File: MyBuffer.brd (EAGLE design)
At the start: 137.5 x 110 mm, 102 parts, among them Q1 BD140, Q2 BD139, Q3 BD140, Q4 BD139, Q5 BD139, Q6 BD139, T10 BD140, T11 BD139, T12 BD140, T13 BD139, T14 BD140, T17 BD139, T18 BD140, T9 BD139

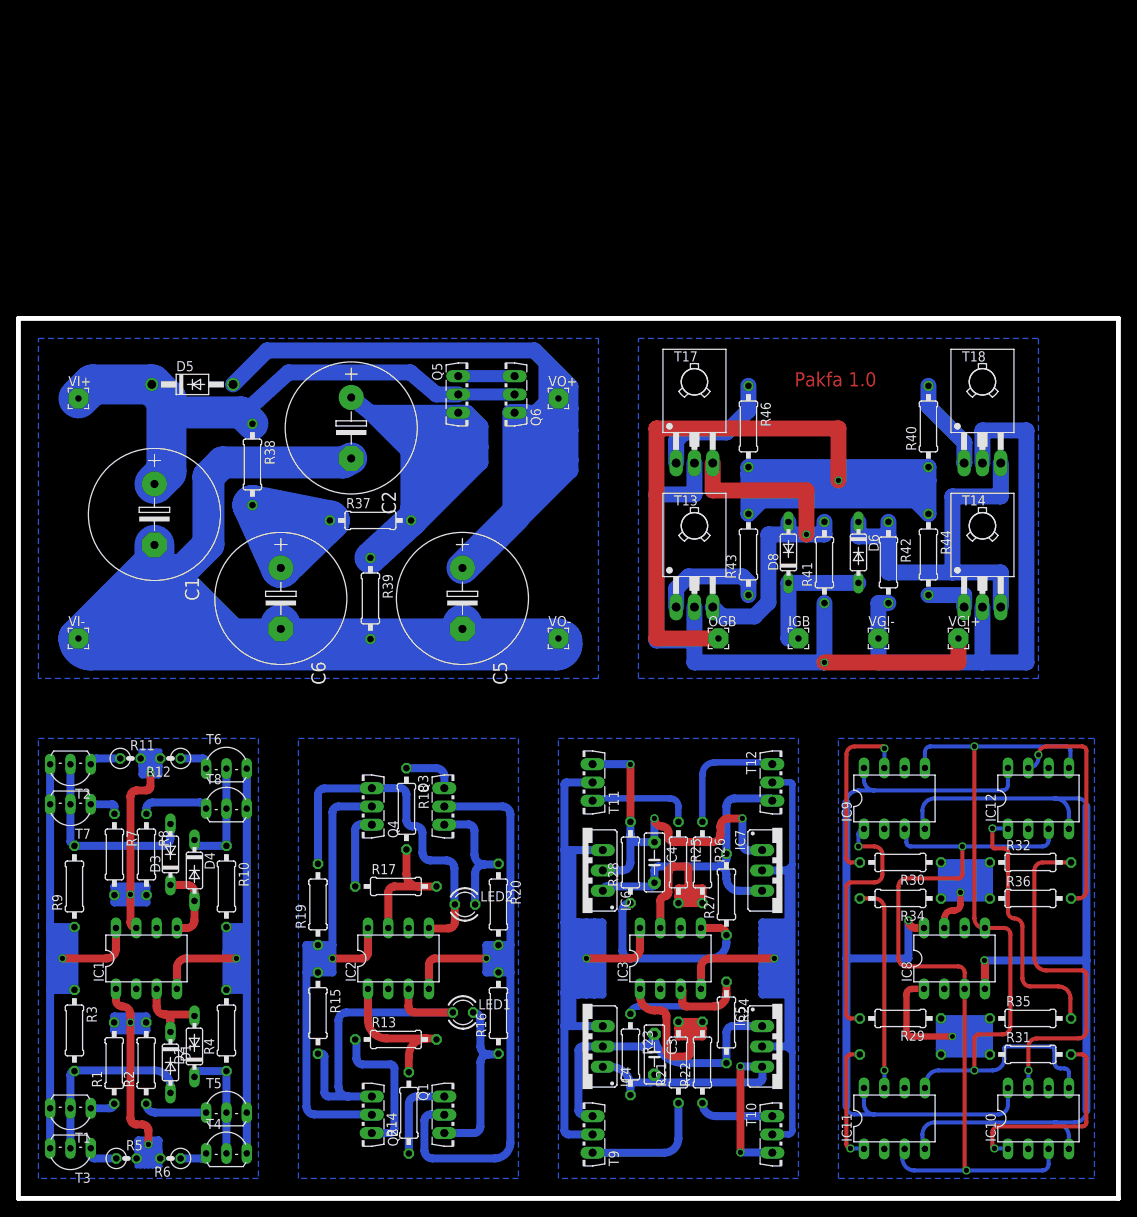
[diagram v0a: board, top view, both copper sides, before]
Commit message: Initial Commit
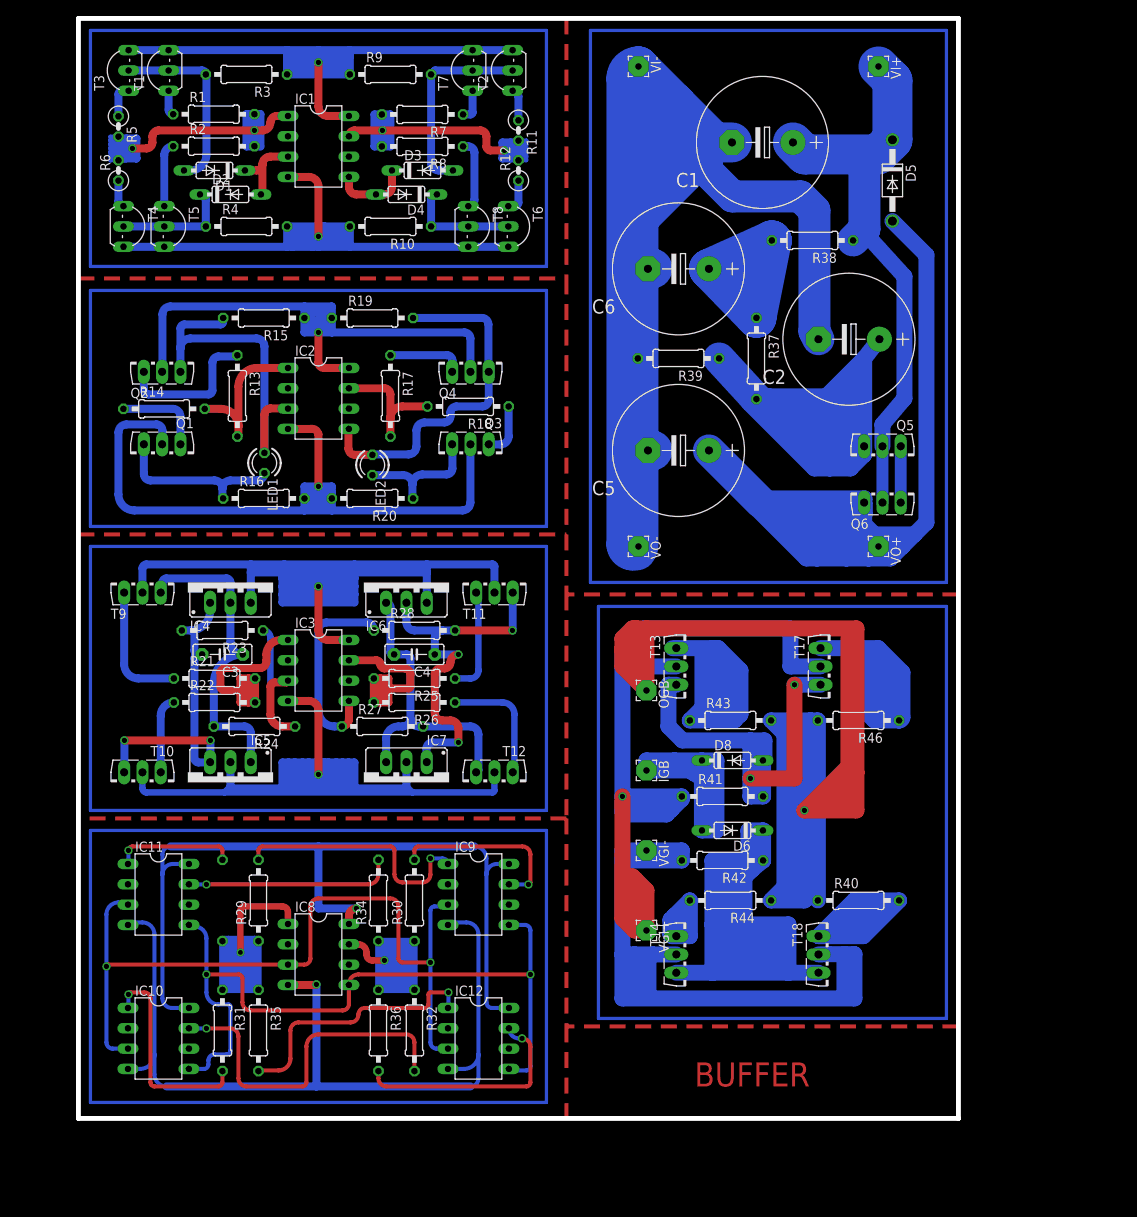
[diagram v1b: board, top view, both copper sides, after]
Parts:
- T13, T17: device transistor-npn:TO126 -> transistor-power:TO126AV
- T14, T18: device transistor-pnp:TO126 -> transistor-power:TO126AV
- moved T3 136.1 mm to (5.00, 131.0), turned to 90 degrees
- moved T1 131.5 mm to (10.0, 131.0), turned to 90 degrees
- moved R5 129.0 mm to (5.00, 124.0), turned to 270 degrees
- moved R6 123.7 mm to (5.00, 118.5), turned to 90 degrees
- moved R3 121.4 mm to (21.0, 130.5), turned to 180 degrees
- moved R1 119.3 mm to (16.9, 125.5), turned to 0 degrees
- moved T4 115.2 mm to (6.90, 111.5), turned to 270 degrees
- moved R2 114.9 mm to (16.9, 121.5), turned to 0 degrees
- moved D1 111.6 mm to (17.0, 118.5), turned to 180 degrees
- moved IC10 110.5 mm to (10.0, 10.0), turned to 270 degrees
- moved T5 109.7 mm to (12.0, 111.5), turned to 270 degrees
- moved R9 108.9 mm to (39.0, 130.5), turned to 0 degrees
- moved VI+ 108.3 mm to (100.0, 131.5), turned to 270 degrees
- moved D2 106.6 mm to (19.0, 115.5), turned to 0 degrees
- moved T7 105.1 mm to (48.0, 131.0), turned to 90 degrees
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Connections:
- net N$42: now also T17.E; no longer T17.1
- net N$44: now also T18.E; no longer T18.1
- net N$45: now also T14.B, T18.B; no longer T14.3, T18.3
- net N$46: now also T13.B, T17.B; no longer T13.3, T17.3
- net N$48: now also T13.C, T17.C; no longer T13.2, T17.2
- net N$50: now also T14.C, T18.C; no longer T14.2, T18.2
- net N$52: now also T13.E; no longer T13.1
- net N$54: now also T14.E; no longer T14.1
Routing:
- net N$61: track 0.00 -> 418.5 mm
- net N$59: track 0.00 -> 227.0 mm
- net N$60: track 0.00 -> 190.0 mm
- net N$58: track 0.00 -> 182.0 mm
- net N$57: track 0.00 -> 180.0 mm
- net N$56: track 0.00 -> 173.0 mm
- net N$55: track 0.00 -> 173.0 mm
- net N$45: track 50.0 -> 129.9 mm
- net N$40: track 166.1 -> 216.8 mm
- net N$42: track 16.5 -> 56.5 mm
- net N$52: track 13.9 -> 53.3 mm
- net N$48: track 82.0 -> 118.3 mm
- net N$44: track 11.5 -> 36.0 mm
- net N$51: track 16.9 -> 39.5 mm
- net N$50: track 72.7 -> 94.6 mm
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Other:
- board size 137.5 x 110 mm -> 110 x 137.5 mm
- board text added: "BUFFER"
- board text removed: "Pakfa 1.0"
